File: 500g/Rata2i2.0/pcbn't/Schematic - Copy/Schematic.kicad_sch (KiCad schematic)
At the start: 47 parts, among them J1 distance 1, J10 start, J11 motor 1, J13 distance 6, J14 line 4, J16 Screw_Terminal_01x07, J19 motor 2, J2 distance 2, J3 distance 3, J4 distance 4, J5 line 1, J6 line 2, J7 Battery, J9 distance 5, SW1 SW_SPDT, SW2 SW_Push, U1 DEV-16771, U2 NRF24L01_Breakout, U3 R-78K5.0-0.5 (vr 5v), U4 R-78K5.0-0.5 (vr 3.3v), U5 motor driver 1, U6 motor driver 2

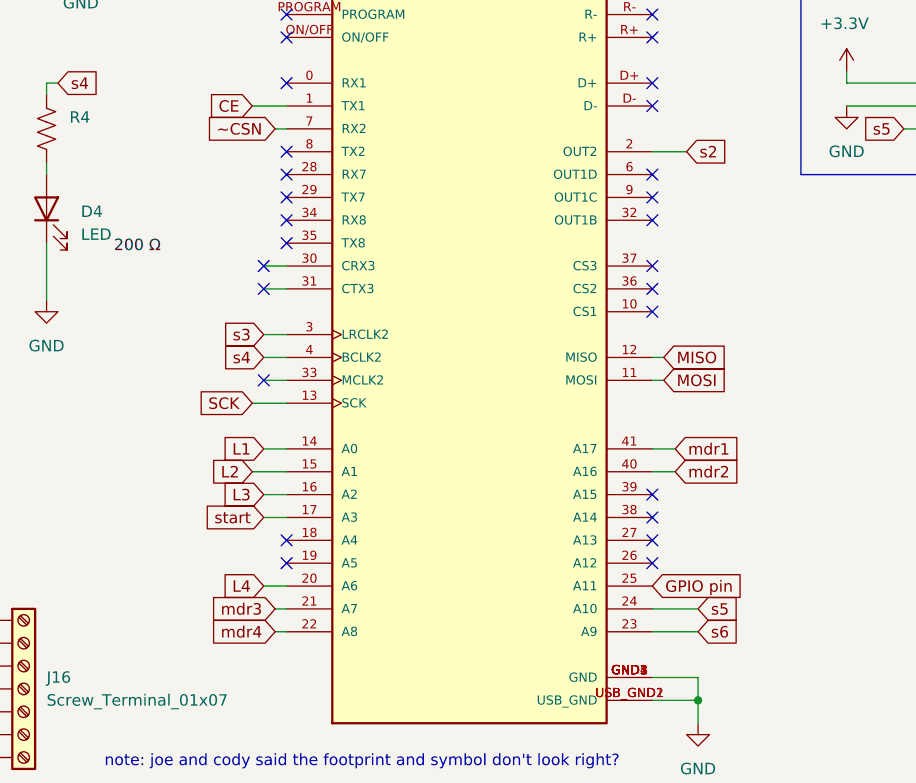
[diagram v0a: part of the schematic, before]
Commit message: Changed motor driver pins
mdr1 - 28
mdr2 - 29
mdr3 - 18
mdr4 - 22
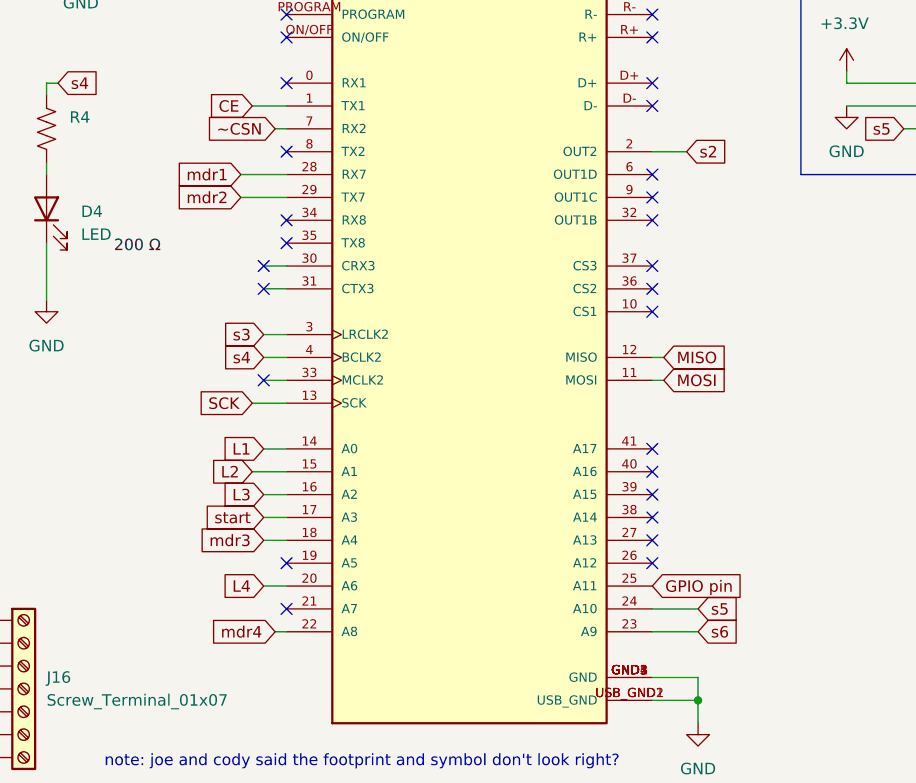
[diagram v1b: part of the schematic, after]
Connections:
- net mdr1: now also U1.28 (RX7); no longer U1.41 (A17)
- net mdr2: now also U1.29 (TX7); no longer U1.40 (A16)
- net mdr3: now also U1.18 (A4); no longer U1.21 (A7)
